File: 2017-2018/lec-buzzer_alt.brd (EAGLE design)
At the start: 62 x 29.5 mm, 26 parts, among them U1 74HC595PW, U2 74HC595PW, U3 DRV2605LDGSR, U4 ATMEGA328P-SUR, U5 74HC595PW, U6 74HC595PW, X1 2X3SHROUDED, X2 MINI-USB-32005-201

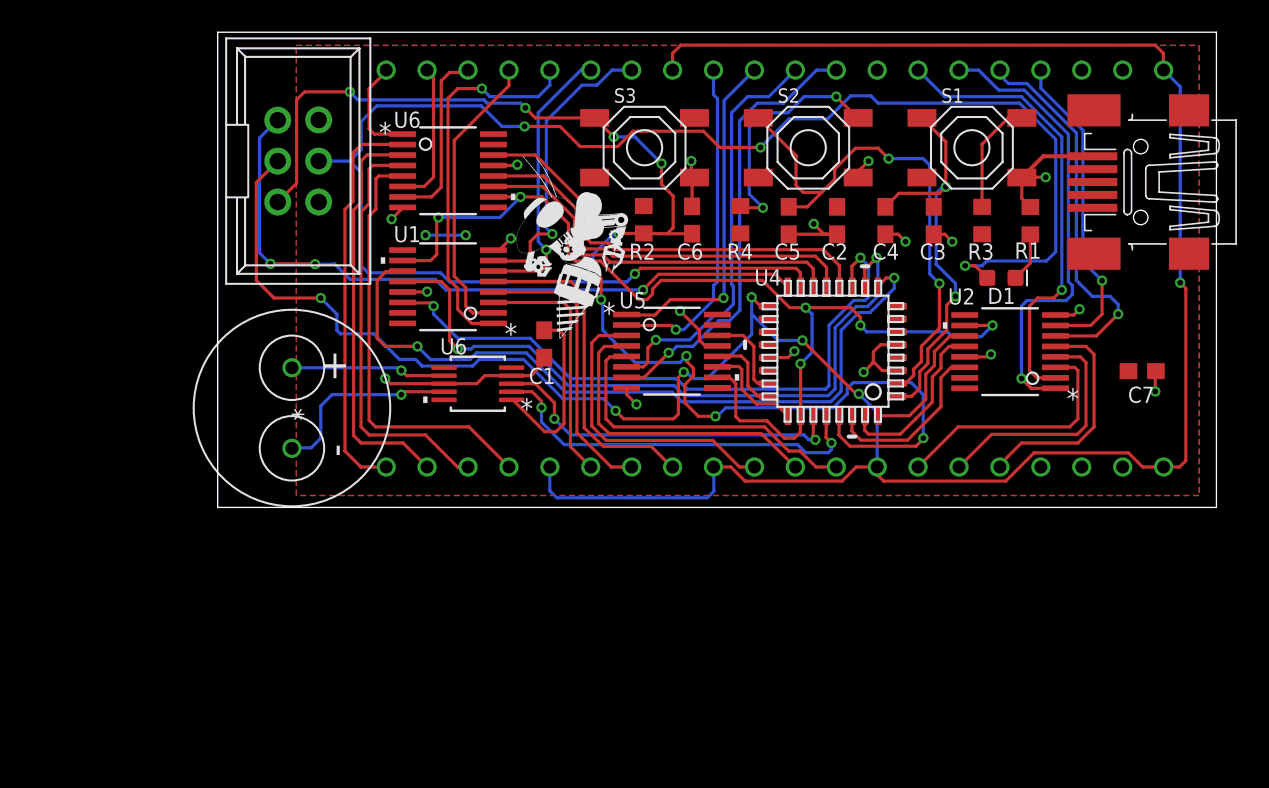
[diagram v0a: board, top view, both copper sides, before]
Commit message: training board v1.1
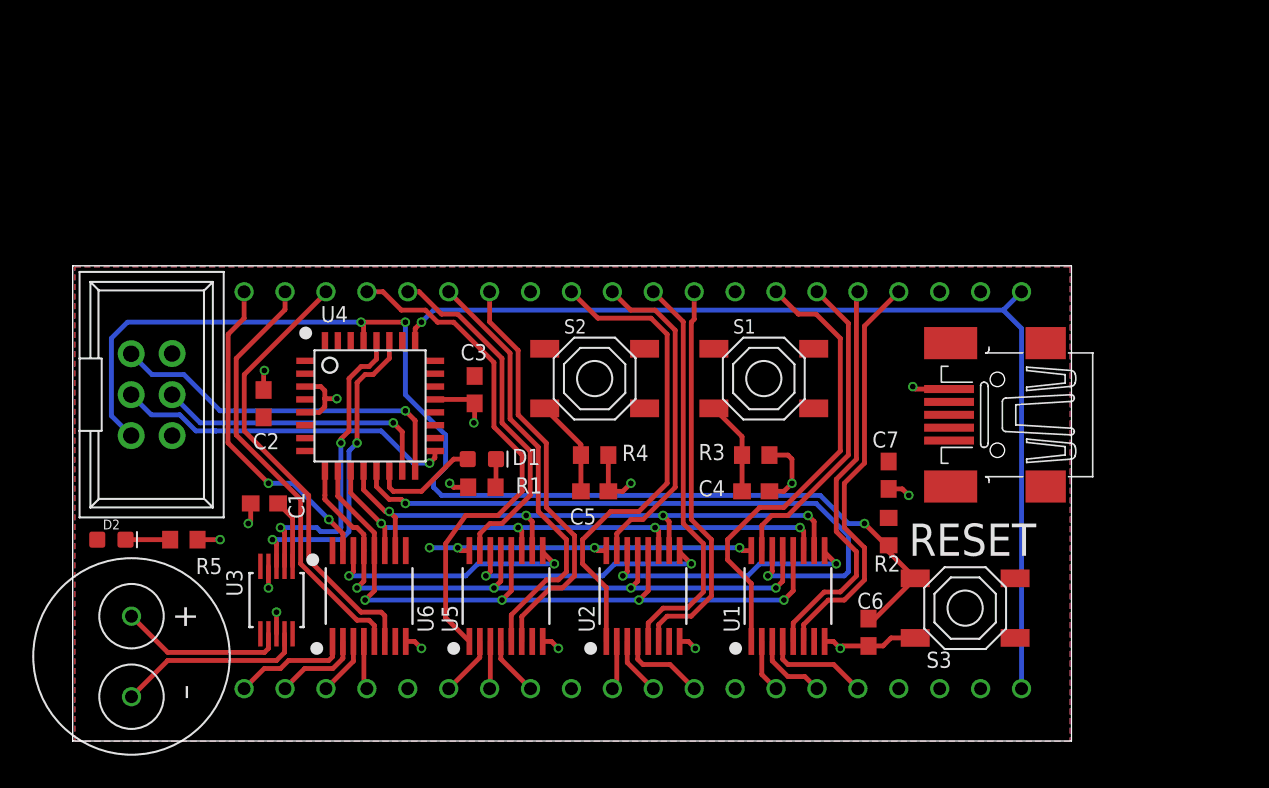
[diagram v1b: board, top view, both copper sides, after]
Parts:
- removed DS1: LCD-S401C39TR, lcd-buzzer:S401C39TR
- added D2: Green, SparkFun-LED:LED-0603
- added LCD1: LCD-S401C39TR, lcd-buzzer:S401C39TR
- added R5: 150, resistor:R0603
- D1: value Yellow -> Blue
- U4: value ATMEGA328P-SUR -> ATMEGA328P-AUR; device lcd-buzzer:ATMEGA328P-AUR-REAL -> lcd-buzzer:ATMEGA328P-AUR
- moved R1 37.9 mm to (25.5, 15.8), turned to 0 degrees
- moved C2 37.4 mm to (11.9, 20.9), turned to 90 degrees
- moved S3 34.8 mm to (55.5, 8.25)
- moved D1 34.2 mm to (25.5, 17.5)
- moved C3 30.4 mm to (25.1, 21.8)
- moved U$1 30.1 mm to (6.20, 7.00), flipped to the bottom
- moved U4 29.0 mm to (18.5, 21.0), turned to 0 degrees
- moved U1 28.5 mm to (44.5, 9.00), turned to 90 degrees
- moved C6 27.8 mm to (49.5, 6.75), turned to 270 degrees
- moved U2 27.4 mm to (35.5, 9.00), turned to 90 degrees
- moved U6 26.9 mm to (18.5, 9.00), turned to 90 degrees
- moved R2 24.6 mm to (50.8, 13.0)
- moved C5 20.7 mm to (32.5, 15.5), turned to 0 degrees
- moved R3 20.2 mm to (42.5, 17.8), turned to 0 degrees
- moved C1 20.0 mm to (12.0, 14.8), turned to 180 degrees
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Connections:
- removed net LCD_RESET: U1.10, U2.10, U4.26, U5.10, U6.10
- removed net N$4: U4.19
- removed net N$5: R4.1, S2.2
- removed net N$7: R3.1, S1.2
- removed net SFT1: U2.14, U4.30
- removed net SFT2: U4.23, U5.14
- removed net SFT3: U1.14, U4.11
- removed net SFT4: U4.12, U6.14
- removed net SHIFT_CLK1: U2.12, U4.31
- removed net SHIFT_CLK2: U4.24, U5.12
- removed net SHIFT_CLK3: U1.12, U4.10
- removed net SHIFT_CLK4: U4.13, U6.12
- removed net STORAGE_CLK1: U2.11, U4.32
- removed net STORAGE_CLK2: U4.25, U5.11
- removed net STORAGE_CLK3: U1.11, U4.9
- removed net STORAGE_CLK4: U4.14, U6.11
- removed net VDD/NC: U3.6
- new net COL: LCD1.28
- new net COM: LCD1.1, LCD1.40, U4.25
- new net DP1: LCD1.8
- new net DP2: LCD1.12
- new net DP3: LCD1.16
- new net LED1: D1.A, U4.14
- new net N$2: D2.C, R5.2
- new net SFT-!OE: U1.13, U2.13, U4.9, U5.13, U6.13
- new net SFT-!RESET: U1.10, U2.10, U4.12, U5.10, U6.10
- new net SFT-CLK: U1.11, U2.11, U4.11, U5.11, U6.11
- new net SFT-LATCH: U1.12, U2.12, U4.10, U5.12, U6.12
- new net SFT1-IN: U1.14, U4.13
- new net SFT2-IN: U1.9, U2.14
- new net SFT3-IN: U2.9, U5.14
- new net SFT4-IN: U5.9, U6.14
- net !BTN2: now also R4.1, S2.4; no longer S2.1, U4.2
- net !BTN3: now also R3.1, S1.4; no longer S1.1, U4.1
- net +5V: now also D2.A, S1.1, S2.1; no longer R3.2, R4.2
- net 1A: now also LCD1.35, U1.15; no longer DS1.P$35, U2.1
- net 1B: now also LCD1.34, U1.1; no longer DS1.P$34, U2.2
- net 1C: now also LCD1.7, U1.2; no longer DS1.P$7, U2.3
- net 1D: now also LCD1.6, U1.3; no longer DS1.P$6, U2.4
- net 1E: now also LCD1.5, U1.4; no longer DS1.P$5, U2.5
- net 1F: now also LCD1.36, U1.5; no longer DS1.P$36, U2.6
- net 1G: now also LCD1.37, U1.6; no longer DS1.P$37, U2.7
- net 2A: now also LCD1.30, U2.15; no longer DS1.P$30, U5.1
- net 2B: now also LCD1.29, U2.1; no longer DS1.P$29, U5.2
- net 2C: now also LCD1.11, U2.2; no longer DS1.P$11, U5.3
- net 2D: now also LCD1.10, U2.3; no longer DS1.P$10, U5.4
- net 2E: now also LCD1.9, U2.4; no longer DS1.P$9, U5.5
- net 2F: now also LCD1.31, U2.5; no longer DS1.P$31, U5.6
- net 2G: now also LCD1.32, U2.6; no longer DS1.P$32, U5.7
- net 3A: now also LCD1.25, U5.15; no longer DS1.P$25, U1.1
- net 3B: now also LCD1.24, U5.1; no longer DS1.P$24, U1.2
- net 3C: now also LCD1.15, U5.2; no longer DS1.P$15, U1.3
- net 3D: now also LCD1.14, U5.3; no longer DS1.P$14, U1.4
- net 3E: now also LCD1.13, U5.4; no longer DS1.P$13, U1.5
- net 3F: now also LCD1.26, U5.5; no longer DS1.P$26, U1.6
- net 3G: now also LCD1.27, U5.6; no longer DS1.P$27, U1.7
- net 4A: now also LCD1.21, U6.15; no longer DS1.P$21, U6.1
- net 4B: now also LCD1.20, U6.1; no longer DS1.P$20, U6.2
- net 4C: now also LCD1.19, U6.2; no longer DS1.P$19, U6.3
- net 4D: now also LCD1.18, U6.3; no longer DS1.P$18, U6.4
- net 4E: now also LCD1.17, U6.4; no longer DS1.P$17, U6.5
- net 4F: now also LCD1.22, U6.5; no longer DS1.P$22, U6.6
- net 4G: now also LCD1.23, U6.6; no longer DS1.P$23, U6.7
- net GND: now also C1.2, R3.2, R4.2, R5.1, S3.4; no longer C1.1, S1.3, S2.3, S3.3, U1.13, U2.13, U5.13, U6.13
- net LRA/ERM+: now also LS1.1; no longer LS1.P$1
- net LRA/ERM-: now also LS1.2; no longer LS1.P$2
- net MOSI: no longer D1.A
- net N$3: now also C1.1; no longer C1.2
- net SCK: no longer DS1.P$1, DS1.P$12, DS1.P$16, DS1.P$28, DS1.P$40, DS1.P$8
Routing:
- net SCK: track 168.1 -> 21.4 mm, vias 7 -> 1
- net MOSI: track 103.0 -> 17.6 mm, vias 4 -> 1
- net LCD_RESET: track 65.7 -> 0.00 mm, vias 6 -> 0
- net COM: track 0.00 -> 63.4 mm, vias 0 -> 1
- net STORAGE_CLK3: track 46.5 -> 0.00 mm, vias 2 -> 0
- net SFT-LATCH: track 0.00 -> 45.1 mm, vias 0 -> 4
- net SHIFT_CLK3: track 43.7 -> 0.00 mm, vias 2 -> 0
- net SFT-!OE: track 0.00 -> 42.1 mm, vias 0 -> 4
- net SFT3: track 40.7 -> 0.00 mm, vias 2 -> 0
- net SFT1-IN: track 0.00 -> 40.6 mm, vias 0 -> 2
- net SFT-!RESET: track 0.00 -> 39.0 mm, vias 0 -> 4
- net SFT-CLK: track 0.00 -> 36.5 mm, vias 0 -> 4
- net !BTN2: track 33.2 -> 6.08 mm, vias 2 -> 0
- net SFT4: track 26.8 -> 0.00 mm
- net SHIFT_CLK4: track 25.4 -> 0.00 mm
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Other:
- board text added: "RESET"
- board text added: "Training v1.1"
- board text removed: "+"
- board text removed: "-"
- board text removed: "1"
- board text removed: "20"
- board text removed: "21"
- board text removed: "U6"
